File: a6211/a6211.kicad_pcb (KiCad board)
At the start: 2 copper layers, 60 x 25 mm, 27 parts, among them J1 Conn_01x02, J2 Conn_01x02, J3 Conn_01x07, J4 Conn_01x05, J5 Conn_01x02, U1 A6211

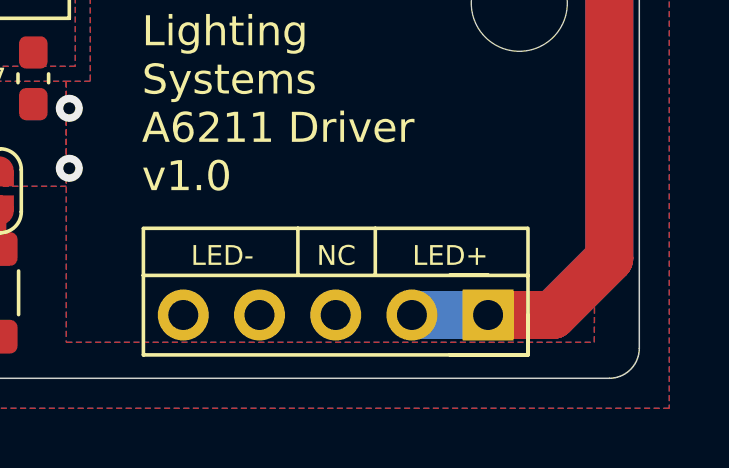
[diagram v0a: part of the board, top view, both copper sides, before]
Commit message: Walkure motherboard production v1.0
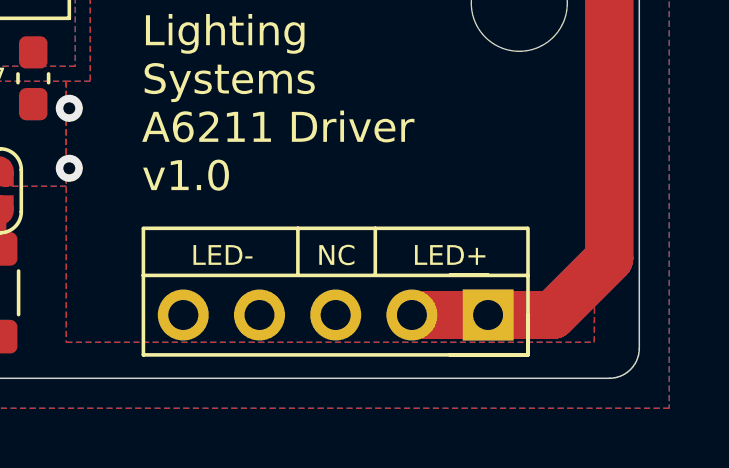
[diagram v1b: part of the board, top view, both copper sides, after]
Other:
- board text added: "Flip these around so ground runs back into the chip See eval board"
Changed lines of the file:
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@@
+		)
+	)
+	(gr_text "Flip these around so ground\nruns back into the chip\nSee eval board"
+		(at 165.56 138.85 0)
+		(layer "Dwgs.User")
+		(effects
+			(font
+				(size 0.66 0.66)
+				(thickness 0.1)
+			)
 		)
 	)
@@
 		(start 190.399999 115.399999)
 		(end 192 117)
+		(width 1.6)
+		(layer "F.Cu")
+		(net 7)
+	)
+	(segment
+		(start 185.42 135.89)
+		(end 187.96 135.89)
 		(width 1.6)
 		(layer "F.Cu")
@@
 		(width 1.6)
 		(layer "B.Cu")
-		(net 7)
-	)
-	(segment
-		(start 187.96 135.89)
-		(end 185.42 135.89)
-		(width 1.6)
-		(layer "B.Cu")

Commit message: A6211 BOM files
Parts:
- D1: value D_Schottky -> Diode
- L1: value L -> Inductor
- R1: value R_US -> 120k
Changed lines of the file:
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@@
 			)
 		)
-		(property "Value" "L"
+		(property "Value" "Inductor"
 			(at 0 6.35 0)
 			(layer "F.Fab")
@@
 			)
 		)
-		(property "Value" "D_Schottky"
+		(property "Value" "Diode"
 			(at 0 4.2 0)
 			(layer "F.Fab")
@@
 			)
 		)
-		(property "Value" "R_US"
+		(property "Value" "120k"
 			(at 0 1.43 0)
 			(layer "F.Fab")
